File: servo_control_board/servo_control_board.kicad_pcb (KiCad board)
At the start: 2 copper layers, 25 parts, among them J1 Conn_01x03_Pin, J2 Conn_01x03_Pin, J3 Conn_01x03_Pin, J4 Conn_01x03_Pin, J5 Conn_01x03_Pin, J6 Conn_01x03_Pin, J7 Conn_01x02_Pin, J8 Conn_01x02_Socket

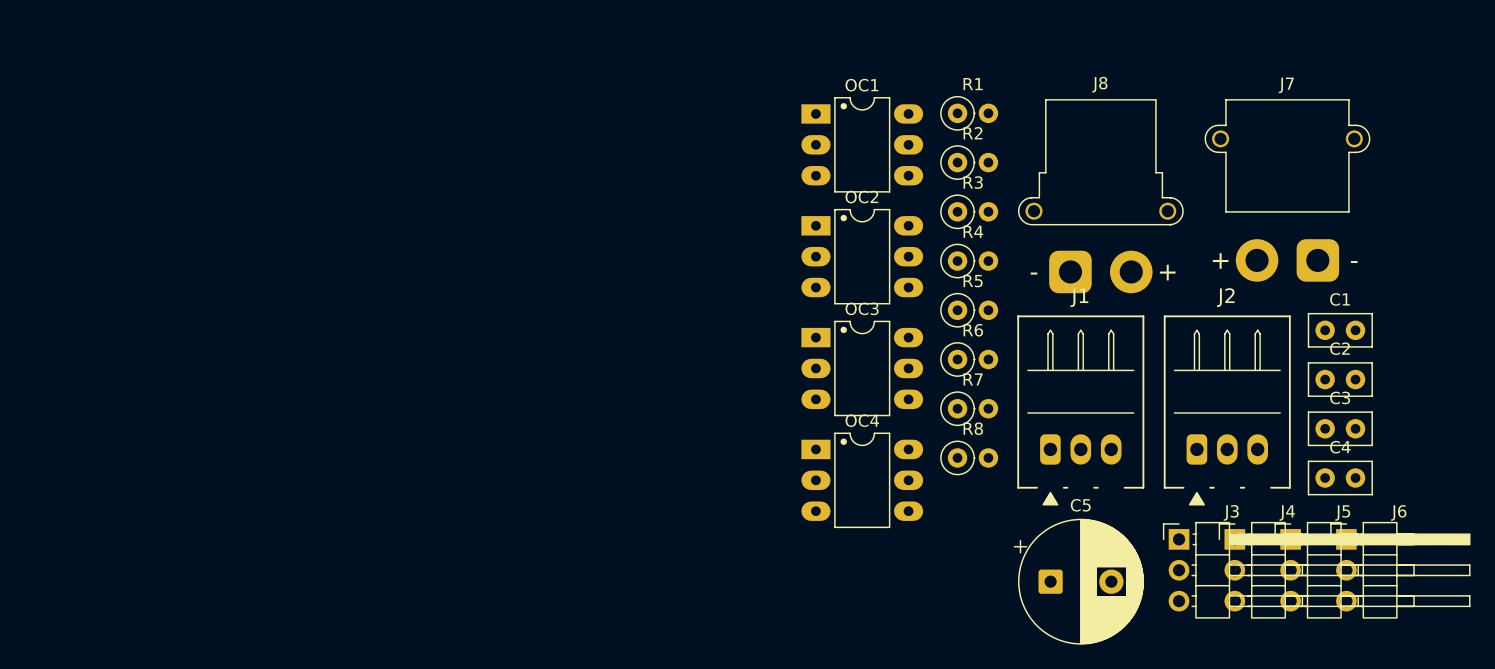
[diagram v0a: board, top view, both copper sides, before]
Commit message: サーボ制御基板　基板完成，ver0.1
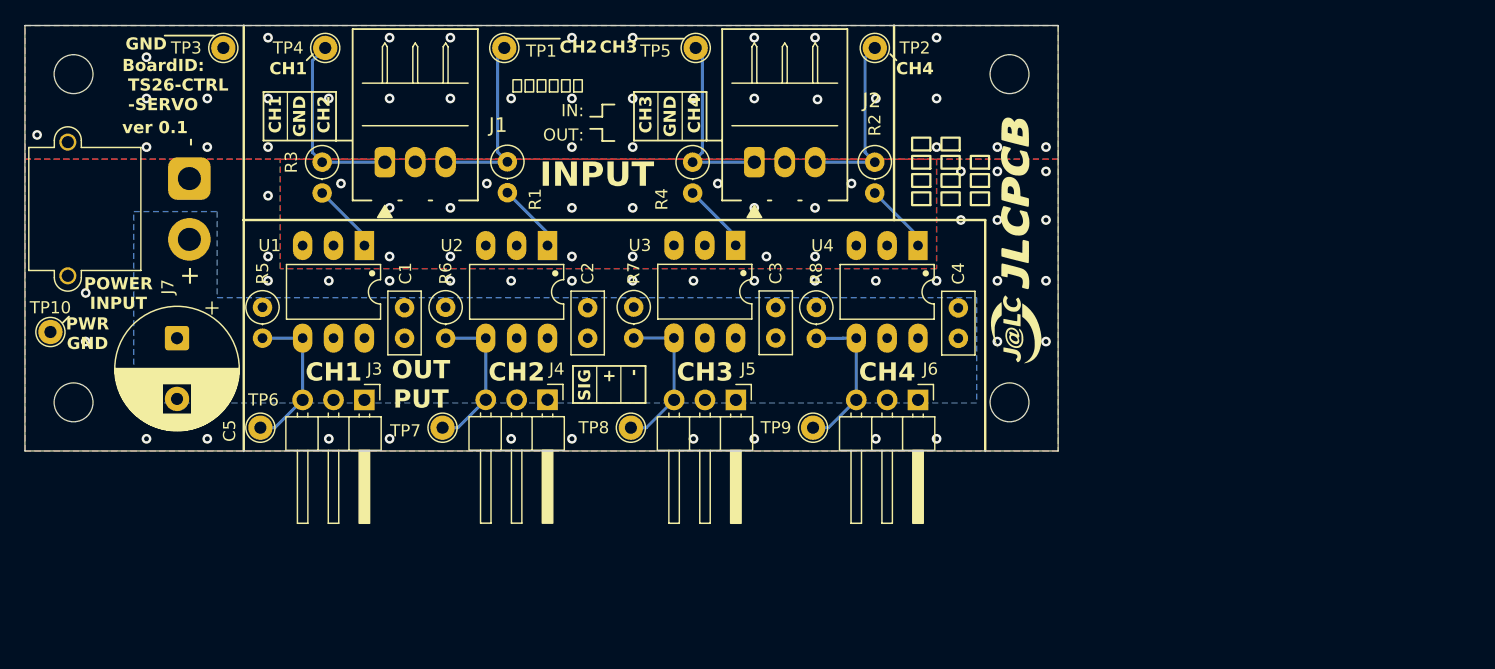
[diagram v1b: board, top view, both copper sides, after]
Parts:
- removed J8: Conn_01x02_Socket, OU_connector:AMASS_XT30PW-F_1x02_P2.50mm_Horizontal
- added G***: LOGO, OU_Picture:JLCPCB_Logo_4x20, F.Cu at (101.5, 37.7)
- added G***: LOGO, OU_Picture:OkaLogo, B.Cu at (69.5, 29.2)
- added REF**: MountingHole_3.2mm_M3, MountingHole:MountingHole_3.2mm_M3, F.Cu at (24.0, 51.0)
- added REF**: MountingHole_3.2mm_M3, MountingHole:MountingHole_3.2mm_M3, F.Cu at (101.0, 51.0)
- added REF**: MountingHole_3.2mm_M3, MountingHole:MountingHole_3.2mm_M3, F.Cu at (24.0, 24.0)
- added REF**: MountingHole_3.2mm_M3, MountingHole:MountingHole_3.2mm_M3, F.Cu at (101.0, 24.0)
- added TP1: TestPoint_Probe, TestPoint:TestPoint_THTPad_D2.0mm_Drill1.0mm, F.Cu at (59.4, 21.8)
- added TP10: TestPoint, TestPoint:TestPoint_THTPad_D2.0mm_Drill1.0mm, F.Cu at (22.1, 45.2)
- added TP2: TestPoint_Probe, TestPoint:TestPoint_THTPad_D2.0mm_Drill1.0mm, F.Cu at (89.9, 21.8)
- added TP3: TestPoint, TestPoint:TestPoint_THTPad_D2.0mm_Drill1.0mm, F.Cu at (36.3, 21.8)
- added TP4: TestPoint_Probe, TestPoint:TestPoint_THTPad_D2.0mm_Drill1.0mm, F.Cu at (44.7, 21.8)
- added TP5: TestPoint_Probe, TestPoint:TestPoint_THTPad_D2.0mm_Drill1.0mm, F.Cu at (75.2, 21.8)
- added TP6: TestPoint_Probe, TestPoint:TestPoint_THTPad_D2.0mm_Drill1.0mm, F.Cu at (39.4, 53.1)
- added TP7: TestPoint_Probe, TestPoint:TestPoint_THTPad_D2.0mm_Drill1.0mm, F.Cu at (54.4, 53.1)
- added TP8: TestPoint_Probe, TestPoint:TestPoint_THTPad_D2.0mm_Drill1.0mm, F.Cu at (69.8, 53.1)
- added TP9: TestPoint_Probe, TestPoint:TestPoint_THTPad_D2.0mm_Drill1.0mm, F.Cu at (84.8, 53.1)
- moved J7 93.1 mm to (33.5, 32.6), turned to 90 degrees
- moved C1 75.8 mm to (51.2, 43.2), turned to -90 degrees
- moved C5 74.6 mm to (32.5, 45.7), turned to -90 degrees
- moved J3 68.0 mm to (47.9, 50.8), turned to -90 degrees
- moved C2 61.0 mm to (66.3, 43.2), turned to -90 degrees
- moved J1 59.6 mm to (49.6, 31.2)
- moved J4 57.7 mm to (63.0, 50.8), turned to -90 degrees
- moved R5 57.2 mm to (39.5, 43.2), turned to -90 degrees
- moved R3 52.4 mm to (44.5, 31.2), turned to -90 degrees
- moved J5 47.1 mm to (78.5, 50.8), turned to -90 degrees
- moved C3 46.3 mm to (81.8, 43.2), turned to -90 degrees
- moved J2 43.4 mm to (80.0, 31.2)
- moved R6 42.3 mm to (54.6, 43.2), turned to -90 degrees
- moved U1 38.7 mm to (47.9, 38.1), turned to -90 degrees
- moved J6 37.1 mm to (93.5, 50.8), turned to -90 degrees
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- renumbered R2 to R1, R4 to R2, R1 to R3, R3 to R4, OC1 to U1, OC2 to U2, OC3 to U3, OC4 to U4
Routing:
- net Net-(J1-Pin_1): track 0.00 -> 15.3 mm
- net Net-(J2-Pin_1): track 0.00 -> 15.0 mm
- net Net-(J1-Pin_3): track 0.00 -> 15.0 mm
- net Net-(J2-Pin_3): track 0.00 -> 15.0 mm
- net Net-(J5-Pin_3): track 0.00 -> 12.9 mm
- net Net-(J4-Pin_3): track 0.00 -> 12.9 mm
- net Net-(J6-Pin_3): track 0.00 -> 12.9 mm
- net Net-(J3-Pin_3): track 0.00 -> 12.8 mm
- net Net-(R2-Pad2): track 0.00 -> 5.79 mm
- net Net-(R4-Pad2): track 0.00 -> 5.77 mm
- net Net-(R3-Pad2): track 0.00 -> 5.76 mm
- net Net-(R1-Pad2): track 0.00 -> 5.71 mm
- net GNDPWR: vias 0 -> 36
- net GND: vias 0 -> 48
- added copper zone on B.Cu, net +SERVO
- added copper zone on B.Cu, net GND
- added copper zone on F.Cu, net GND
- added copper zone on B.Cu, net GNDPWR
- added copper zone on F.Cu, net GNDPWR
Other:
- board outline added: 85 x 35 mm
- board text added: "+"
- board text added: "-"
- board text added: "2026/09/24 Designed by E.Yoshioka"
- board text added: "BoardID: TS26-CTRL -SERVO"
- board text added: "CH1"
- board text added: "CH2"
- board text added: "CH3"
- board text added: "CH4"
- board text added: "GND"
- board text added: "IN:"
- board text added: "INPUT"
- board text added: "No."
- board text added: "OUT PUT"
- board text added: "OUT:"
- board text added: "POWER INPUT"
- board text added: "PWR GND"
- board text added: "SIG"
- board text added: "ver 0.1"
- board text added: "岡山大学 ロボット 研究会"
- board text added: "注：反転出力"
